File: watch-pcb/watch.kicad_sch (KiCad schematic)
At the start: 31 parts, among them J1 Conn_01x02, J2 Conn_01x08, J3 Conn_01x02_Female, J4 Conn_01x08, SW1 EVQ-P4MB3K, SW2 EVQ-P4MB3K, SW3 EVQ-P4MB3K, SW4 EVQ-P4MB3K, U1 NCP161, U2 ATmega328-A, U3 RFM69HCW, U4 PCF85263ATT

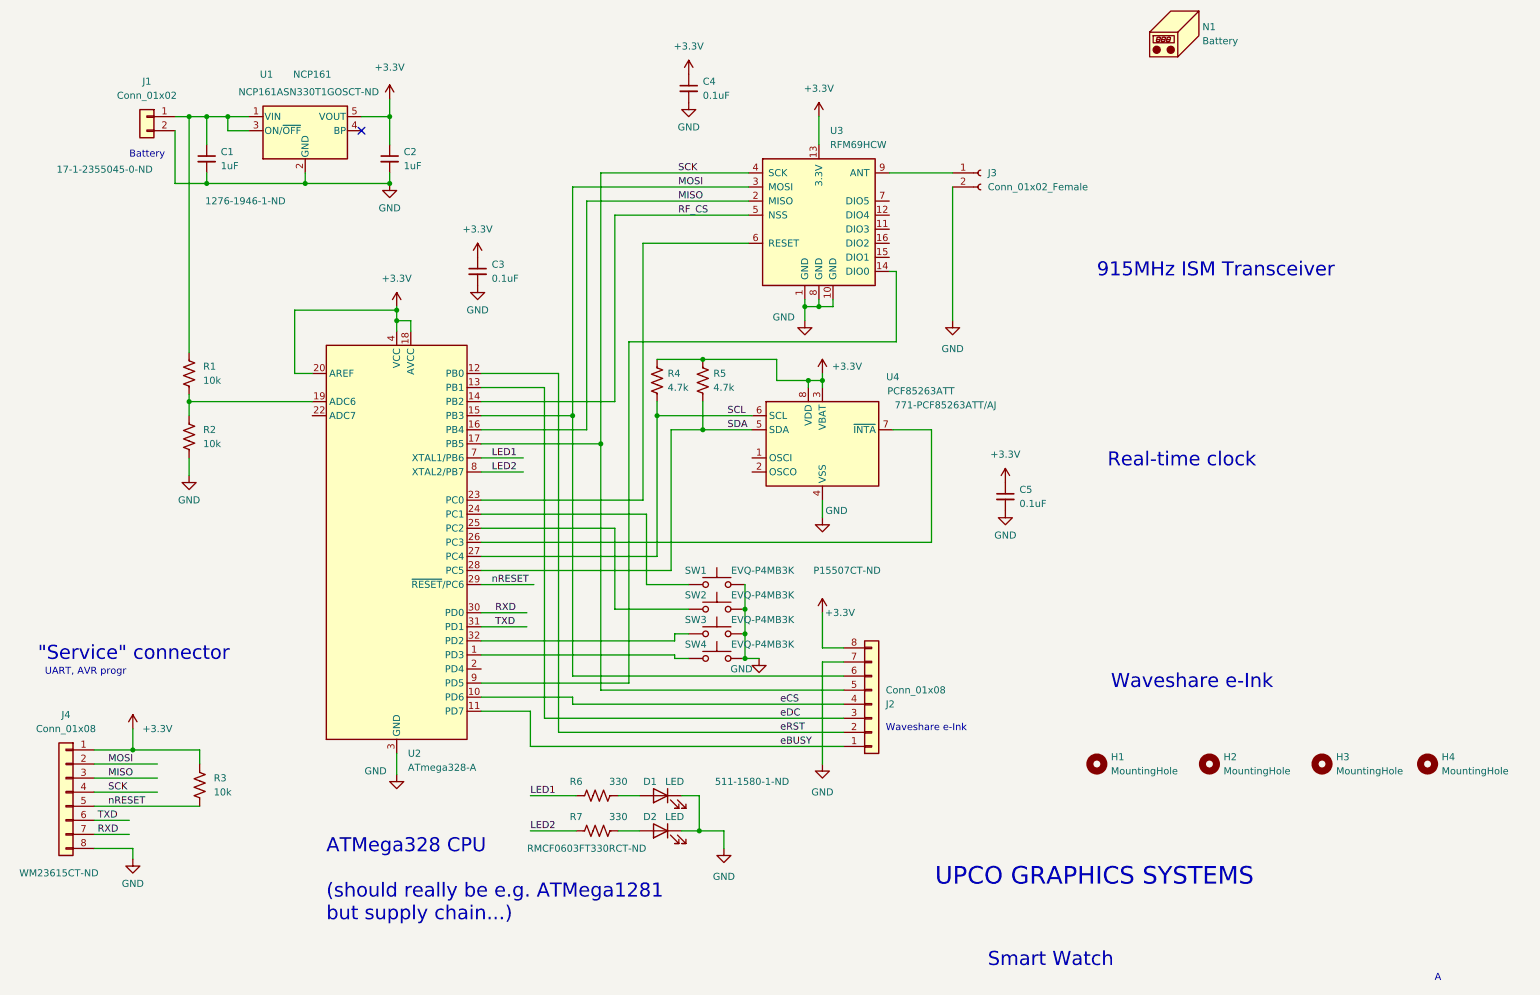
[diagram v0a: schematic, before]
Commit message: tweak software, schem notes
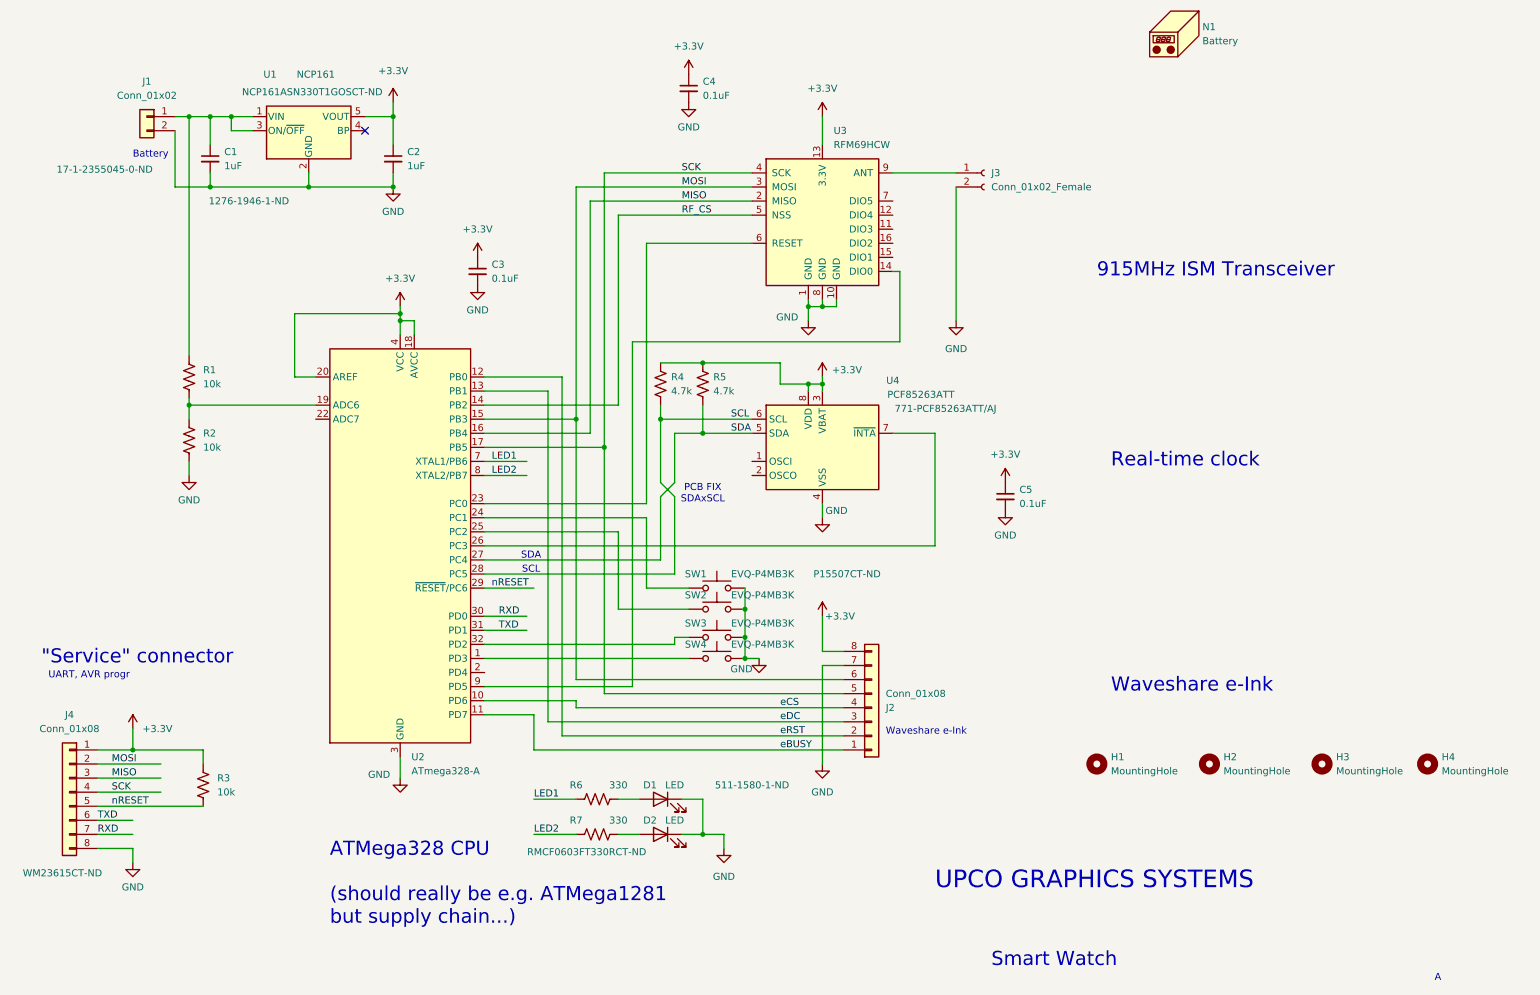
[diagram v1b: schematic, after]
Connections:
- net SCL: now also U2.28 (PC5); no longer U2.27 (PC4)
- net SDA: now also U2.27 (PC4); no longer U2.28 (PC5)
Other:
- note added: "PCB FIX SDAxSCL"
- note added: "SCL"
- note added: "SDA"
- moved on the sheet: C1, C2, D1, D2, J2, J3, J4, R1, R2, R3, R4, R5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
